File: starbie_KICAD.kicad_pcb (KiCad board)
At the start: 2 copper layers, 93.3 x 74.9 mm, 7 parts, among them J1 Conn_01x04_Pin, J2 Conn_01x08_Pin, SW1 SW_Push, SW2 SW_Push, U1 DHT11, U2 XIAO-ESP32-C3-SMD

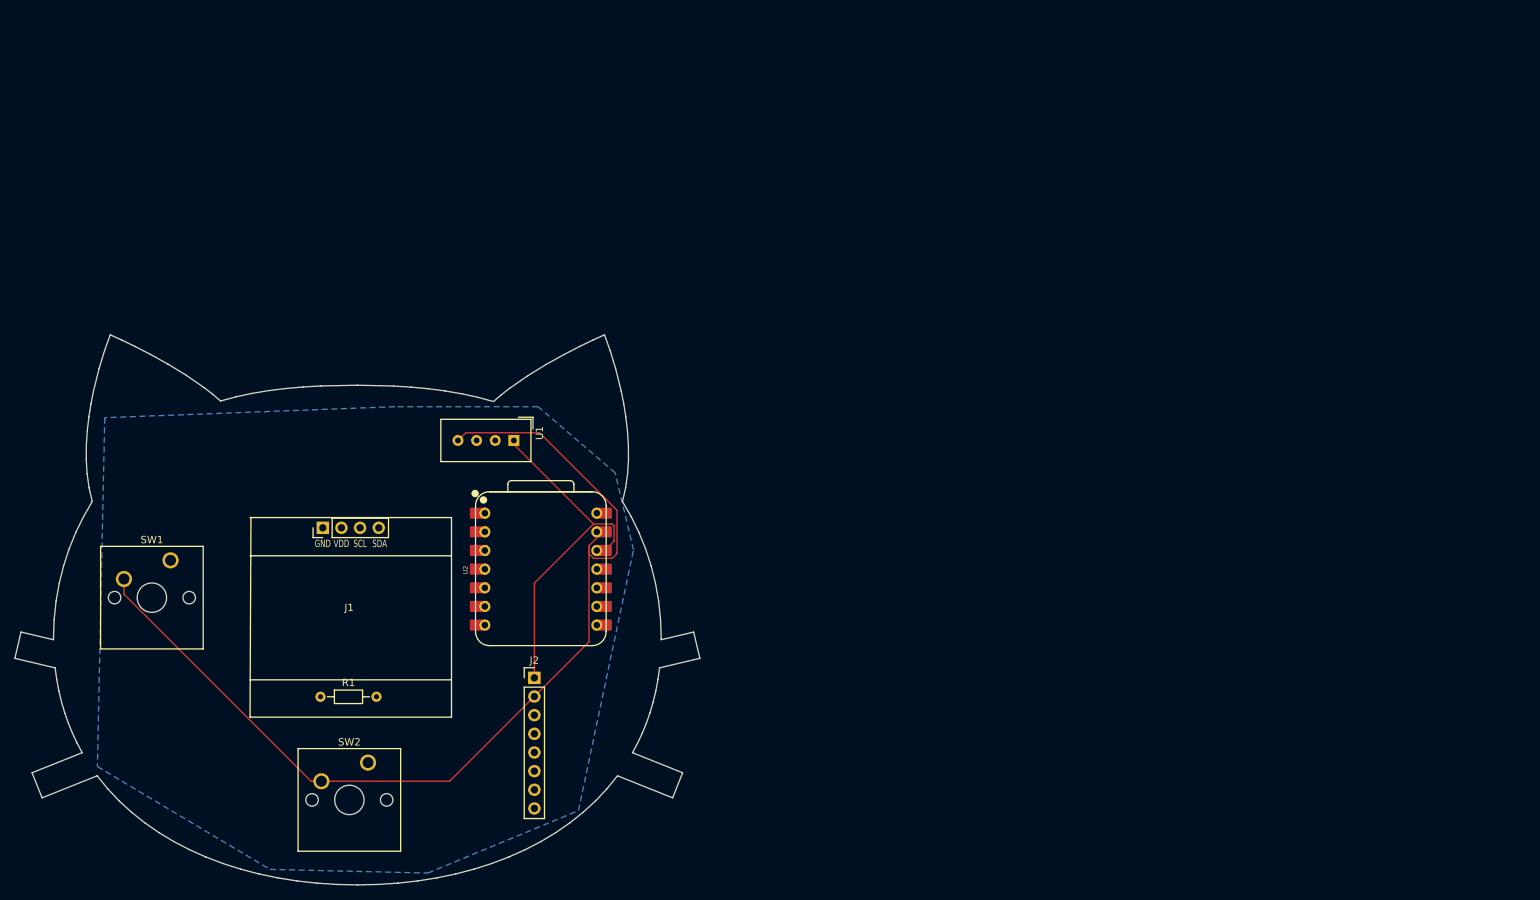
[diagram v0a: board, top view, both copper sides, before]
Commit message: Autosave
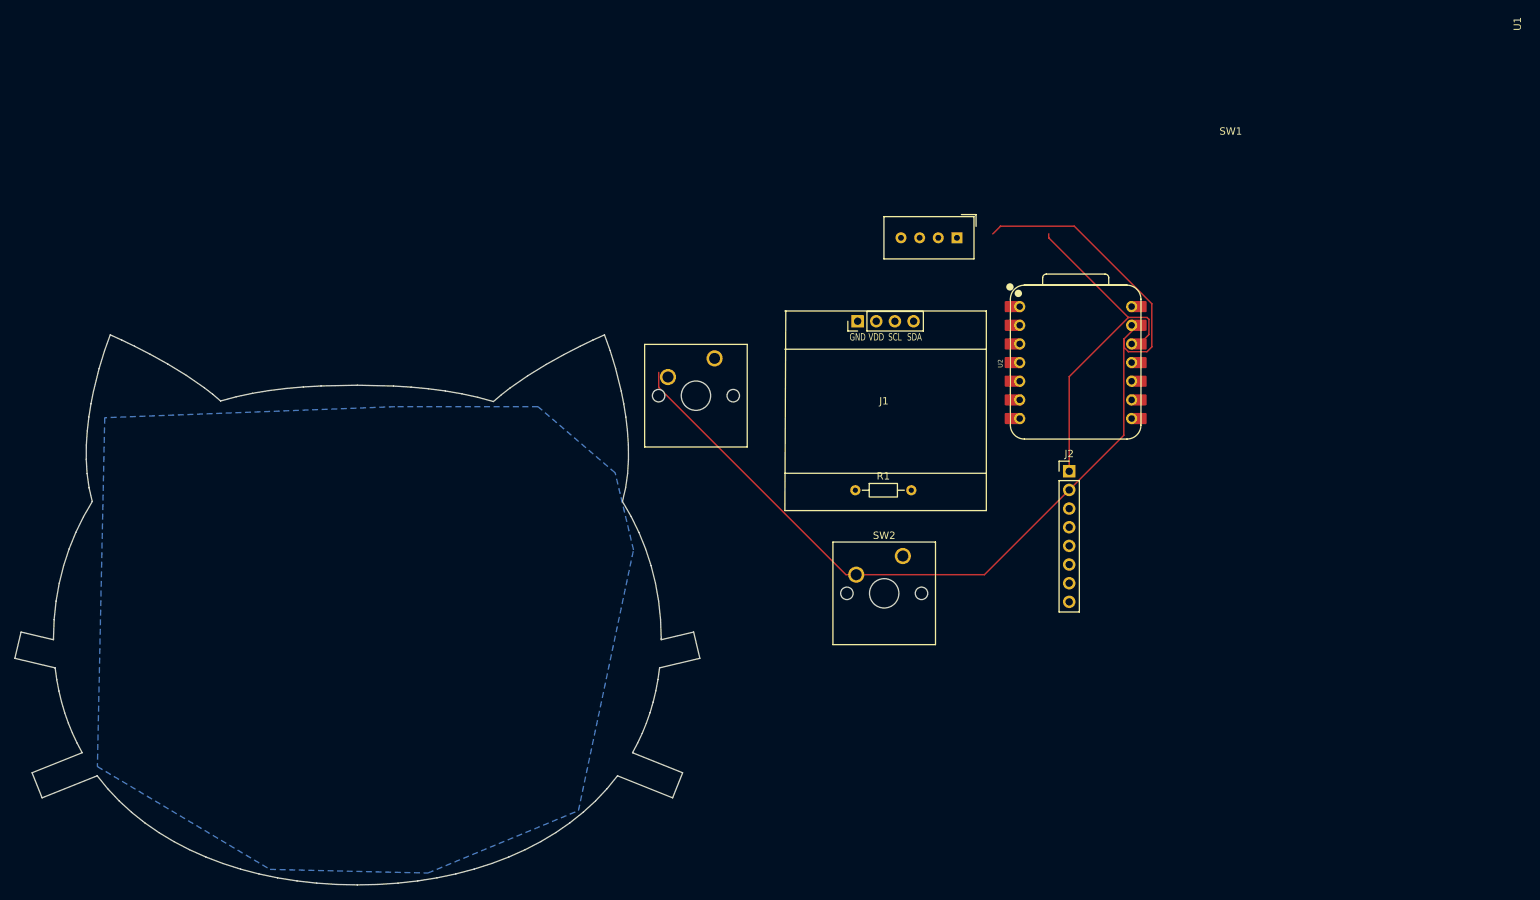
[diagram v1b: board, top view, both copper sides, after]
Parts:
- moved SW1 79.0 mm to (220.0, 44.9)
- moved J1 78.1 mm to (243.3, 39.9)
- moved J2 78.1 mm to (268.3, 60.3)
- moved R1 78.1 mm to (239.2, 62.9)
- moved SW2 78.1 mm to (245.7, 71.8)
- moved U2 78.1 mm to (269.2, 45.5)
- moved U1 66.3 mm to (253.0, 28.5)
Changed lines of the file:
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@@
 	(footprint "Resistor_THT:R_Axial_DIN0204_L3.6mm_D1.6mm_P7.62mm_Horizontal"
 		(layer "F.Cu")
-		(at 166.38 91)
+		(at 239.204 62.873)
 		(descr "Resistor, Axial_DIN0204 series, Axial, Horizontal, pin pitch=7.62mm, 0.167W, length*diameter=3.6*1.6mm^2, http://cdn-reichelt.de/documents/datenblatt/B400/1_4W%23YAG.pdf")
 		(tags "Resistor Axial_DIN0204 series Axial Horizontal pin pitch 7.62mm 0.167W length 3.6mm diameter 1.6mm")
@@
 	(footprint "Imported Parts:XIAO-ESP32-C6-DIP"
 		(layer "F.Cu")
-		(at 196.38 73.62 90)
+		(at 269.204 45.493 90)
 		(property "Reference" "U2"
 			(at -0.125 -10.25 90)
@@
 	(footprint "Button_Switch_Keyboard:SW_Cherry_MX_1.00u_PCB"
 		(layer "F.Cu")
-		(at 172.85 99.96)
+		(at 245.674 71.833)
 		(descr "Cherry MX keyswitch, 1.00u, PCB mount, http://cherryamericas.com/wp-content/uploads/2014/12/mx_cat.pdf")
 		(tags "Cherry MX keyswitch 1.00u PCB")
@@
 	(footprint "Button_Switch_Keyboard:SW_Cherry_MX_1.00u_PCB"
 		(layer "F.Cu")
-		(at 145.96 72.42)
+		(at 220.04 44.92)
 		(descr "Cherry MX keyswitch, 1.00u, PCB mount, http://cherryamericas.com/wp-content/uploads/2014/12/mx_cat.pdf")
 		(tags "Cherry MX keyswitch 1.00u PCB")
 		(property "Reference" "SW1"
-			(at -2.54 -2.794 0)
+			(at 70.284 -30.921 0)
 			(layer "F.SilkS")
 			(effects
@@
 		)
 		(property "Value" "SW_Push"
-			(at -2.54 12.954 0)
+			(at 70.284 -15.173 0)
 			(layer "F.Fab")
 			(effects
@@
 		)
 		(fp_text user "${REFERENCE}"
-			(at -2.54 -2.794 0)
+			(at 70.284 -30.921 0)
 			(layer "F.Fab")
 			(effects
@@
 	(footprint "Imported Parts:Display_128x64_096_I2C"
 		(layer "F.Cu")
-		(at 170.5 67.992)
+		(at 243.324 39.865)
 		(descr "Display 0.96\" OLED 128x64 pixel with SSD1306 controller and I2C interface")
 		(tags "display OLED SSD1306 128x64")
@@
 	(footprint "Sensor:Aosong_DHT11_5.5x12.0_P2.54mm"
 		(layer "F.Cu")
-		(at 192.7125 56.0975 -90)
+		(at 253.04 28.5 -90)
 		(descr "Temperature and humidity module, http://akizukidenshi.com/download/ds/aosong/DHT11.pdf")
 		(tags "Temperature and humidity module")
 		(property "Reference" "U1"
-			(at -1 -3.5 90)
+			(at -29.127 -76.324 90)
 			(layer "F.SilkS")
 			(effects
@@
 		)
 		(property "Value" "DHT11"
-			(at 0 11.3 90)
+			(at -28.127 -61.524 90)
 			(layer "F.Fab")
 			(effects
@@
 		)
 		(fp_text user "${REFERENCE}"
-			(at 0 3.81 90)
+			(at -28.127 -69.014 90)
 			(layer "F.Fab")
 			(effects
@@
 	(footprint "Connector_PinHeader_2.54mm:PinHeader_1x08_P2.54mm_Vertical"
 		(layer "F.Cu")
-		(at 195.5 88.42)
+		(at 268.324 60.293)
 		(descr "Through hole straight pin header, 1x08, 2.54mm pitch, single row")
 		(tags "Through hole pin header THT 1x08 2.54mm single row")
@@
 	)
 	(segment
-		(start 205.07763 71.08)
-		(end 204 71.08)
+		(start 277.90163 42.953)
+		(end 276.824 42.953)
 		(width 0.2)
 		(layer "F.Cu")
@@
 	)
 	(segment
-		(start 206.351 69.80663)
-		(end 205.07763 71.08)
+		(start 279.175 41.67963)
+		(end 277.90163 42.953)
 		(width 0.2)
 		(layer "F.Cu")
@@
 	)
 	(segment
-		(start 192.7125 56.630395)
-		(end 203.560105 67.478)
+		(start 265.5365 28.503395)
+		(end 276.384105 39.351)
 		(width 0.2)
 		(layer "F.Cu")
@@
 	)
 	(segment
-		(start 206.351 67.738786)
-		(end 206.351 69.80663)
+		(start 279.175 39.611786)
+		(end 279.175 41.67963)
 		(width 0.2)
 		(layer "F.Cu")
@@
 	)
 	(segment
-		(start 195.5 88.42)
-		(end 195.5 88.5)
+		(start 268.324 60.293)
+		(end 268.324 60.373)
 		(width 0.2)
 		(layer "F.Cu")
@@
 	)
 	(segment
-		(start 206.090214 67.478)
-		(end 206.351 67.738786)
+		(start 278.914214 39.351)
+		(end 279.175 39.611786)
 		(width 0.2)
 		(layer "F.Cu")
@@
 	)
 	(segment
-		(start 195.5 88.42)
-		(end 195.5 75.538105)
+		(start 268.324 60.293)
+		(end 268.324 47.411105)
 		(width 0.2)
 		(layer "F.Cu")
@@
 	)
 	(segment
-		(start 203.560105 67.478)
-		(end 206.090214 67.478)
+		(start 276.384105 39.351)
+		(end 278.914214 39.351)
 		(width 0.2)
 		(layer "F.Cu")
@@
 	)
 	(segment
-		(start 195.5 75.538105)
-		(end 203.560105 67.478)
+		(start 268.324 47.411105)
+		(end 276.384105 39.351)
 		(width 0.2)
 		(layer "F.Cu")
@@
 	)
 	(segment
-		(start 192.7125 56.0975)
-		(end 192.7125 56.630395)
+		(start 265.5365 27.9705)
+		(end 265.5365 28.503395)
 		(width 0.2)
 		(layer "F.Cu")
@@
 	)
 	(segment
-		(start 195.5 90.96)
-		(end 202.938 83.522)
+		(start 268.324 62.833)
+		(end 275.762 55.395)
 		(width 0.2)
 		(layer "F.Cu")
@@
 	)
 	(segment
-		(start 206.751 71.481214)
-		(end 206.090214 72.142)
+		(start 279.575 43.354214)
+		(end 278.914214 44.015)
 		(width 0.2)
 		(layer "F.Cu")
@@
 	)
 	(segment
-		(start 196.199714 55.0475)
-		(end 206.751 65.598786)
+		(start 269.023714 26.9205)
+		(end 279.575 37.471786)
 		(width 0.2)
 		(layer "F.Cu")
@@
 	)
 	(segment
-		(start 206.090214 72.142)
-		(end 203.560105 72.142)
+		(start 278.914214 44.015)
+		(end 276.384105 44.015)
 		(width 0.2)
 		(layer "F.Cu")
@@
 	)
 	(segment
-		(start 206.751 65.598786)
-		(end 206.751 71.481214)
+		(start 279.575 37.471786)
+		(end 279.575 43.354214)
 		(width 0.2)
 		(layer "F.Cu")
@@
 	)
 	(segment
-		(start 139.61 77.013402)
-		(end 165.096598 102.5)
+		(start 212.434 48.886402)
+		(end 237.920598 74.373)
 		(width 0.2)
 		(layer "F.Cu")
@@
 	)
 	(segment
-		(start 166.5 102.5)
-		(end 183.96 102.5)
+		(start 239.324 74.373)
+		(end 256.784 74.373)
 		(width 0.2)
 		(layer "F.Cu")
@@
 	)
 	(segment
-		(start 185.0925 56.0975)
-		(end 186.1425 55.0475)
+		(start 257.9165 27.9705)
+		(end 258.9665 26.9205)
 		(width 0.2)
 		(layer "F.Cu")
@@
 	)
 	(segment
-		(start 202.938 70.437)
-		(end 204.835 68.54)
+		(start 275.762 42.31)
+		(end 277.659 40.413)
 		(width 0.2)
 		(layer "F.Cu")
@@
 	)
 	(segment
-		(start 203.560105 72.142)
-		(end 202.938 71.519895)
+		(start 276.384105 44.015)
+		(end 275.762 43.392895)
 		(width 0.2)
 		(layer "F.Cu")
@@
 	)
 	(segment
-		(start 183.96 102.5)
-		(end 195.5 90.96)
+		(start 256.784 74.373)
+		(end 268.324 62.833)
 		(width 0.2)
 		(layer "F.Cu")
@@
 	)
 	(segment
-		(start 186.1425 55.0475)
-		(end 196.199714 55.0475)
+		(start 258.9665 26.9205)
+		(end 269.023714 26.9205)
 		(width 0.2)
 		(layer "F.Cu")
@@
 	)
 	(segment
-		(start 139.61 74.96)
-		(end 139.61 77.013402)
+		(start 212.434 46.833)
+		(end 212.434 48.886402)
 		(width 0.2)
 		(layer "F.Cu")
@@
 	)
 	(segment
-		(start 165.096598 102.5)
-		(end 166.5 102.5)
+		(start 237.920598 74.373)
+		(end 239.324 74.373)
 		(width 0.2)
 		(layer "F.Cu")
@@
 	)
 	(segment
-		(start 202.938 83.522)
-		(end 202.938 70.437)
+		(start 275.762 55.395)
+		(end 275.762 42.31)
 		(width 0.2)
 		(layer "F.Cu")
@@
 	)
 	(segment
-		(start 202.938 71.519895)
-		(end 202.938 70.437)
+		(start 275.762 43.392895)
+		(end 275.762 42.31)
 		(width 0.2)
 		(layer "F.Cu")
